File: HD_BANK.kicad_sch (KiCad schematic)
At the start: 1 part, among them J8 DF40HC(3.0)-120DS

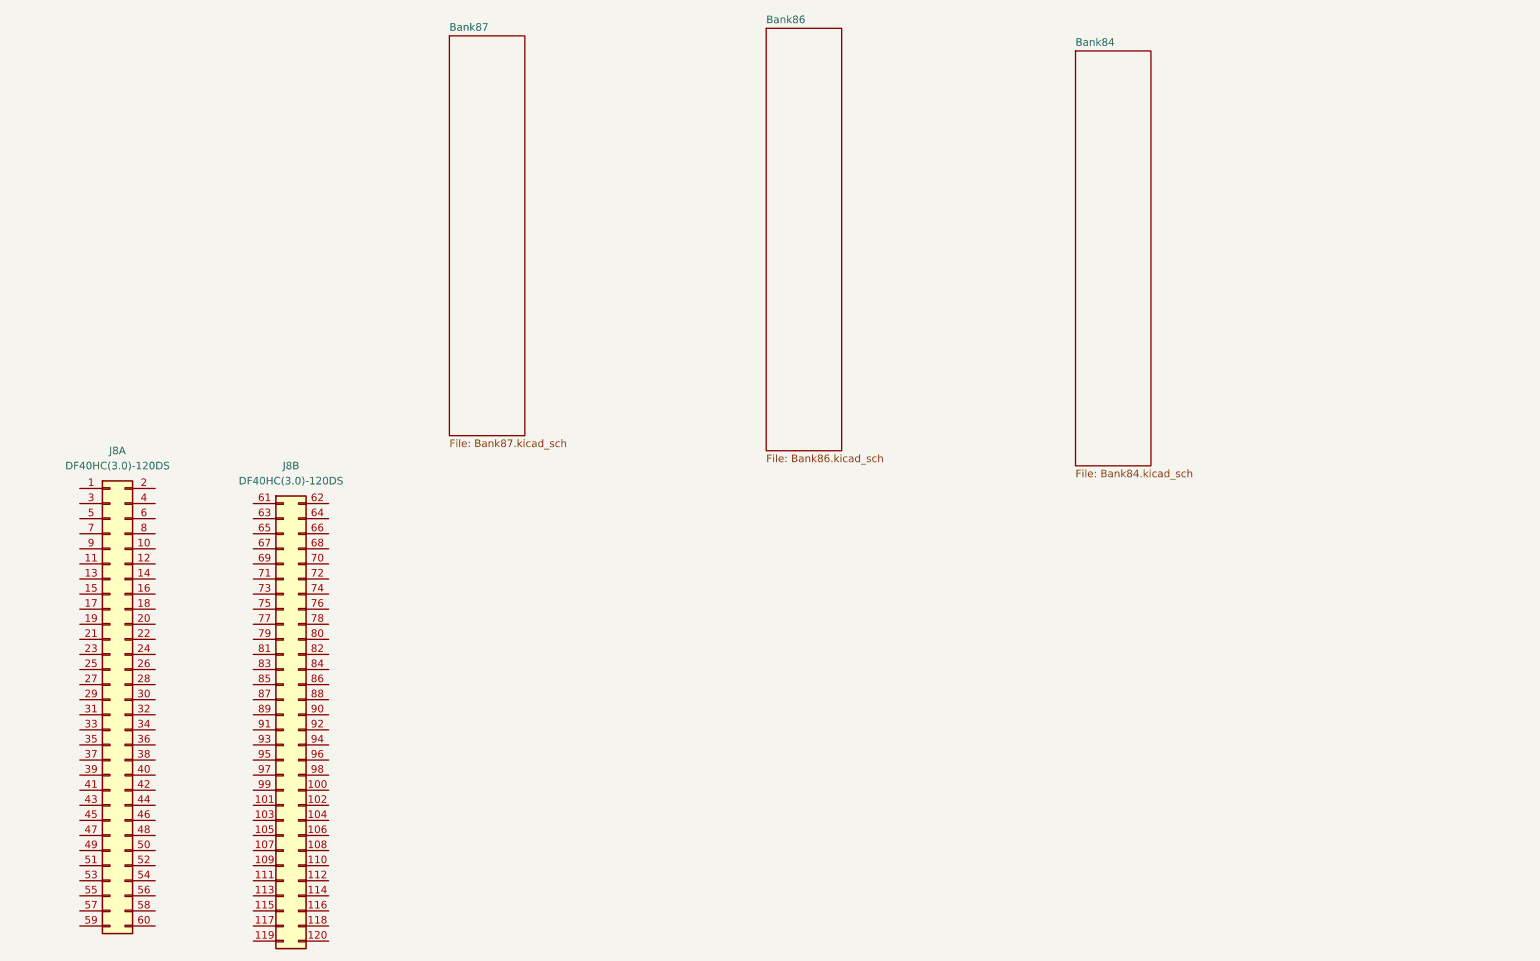
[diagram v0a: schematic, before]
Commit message: finishing schematic
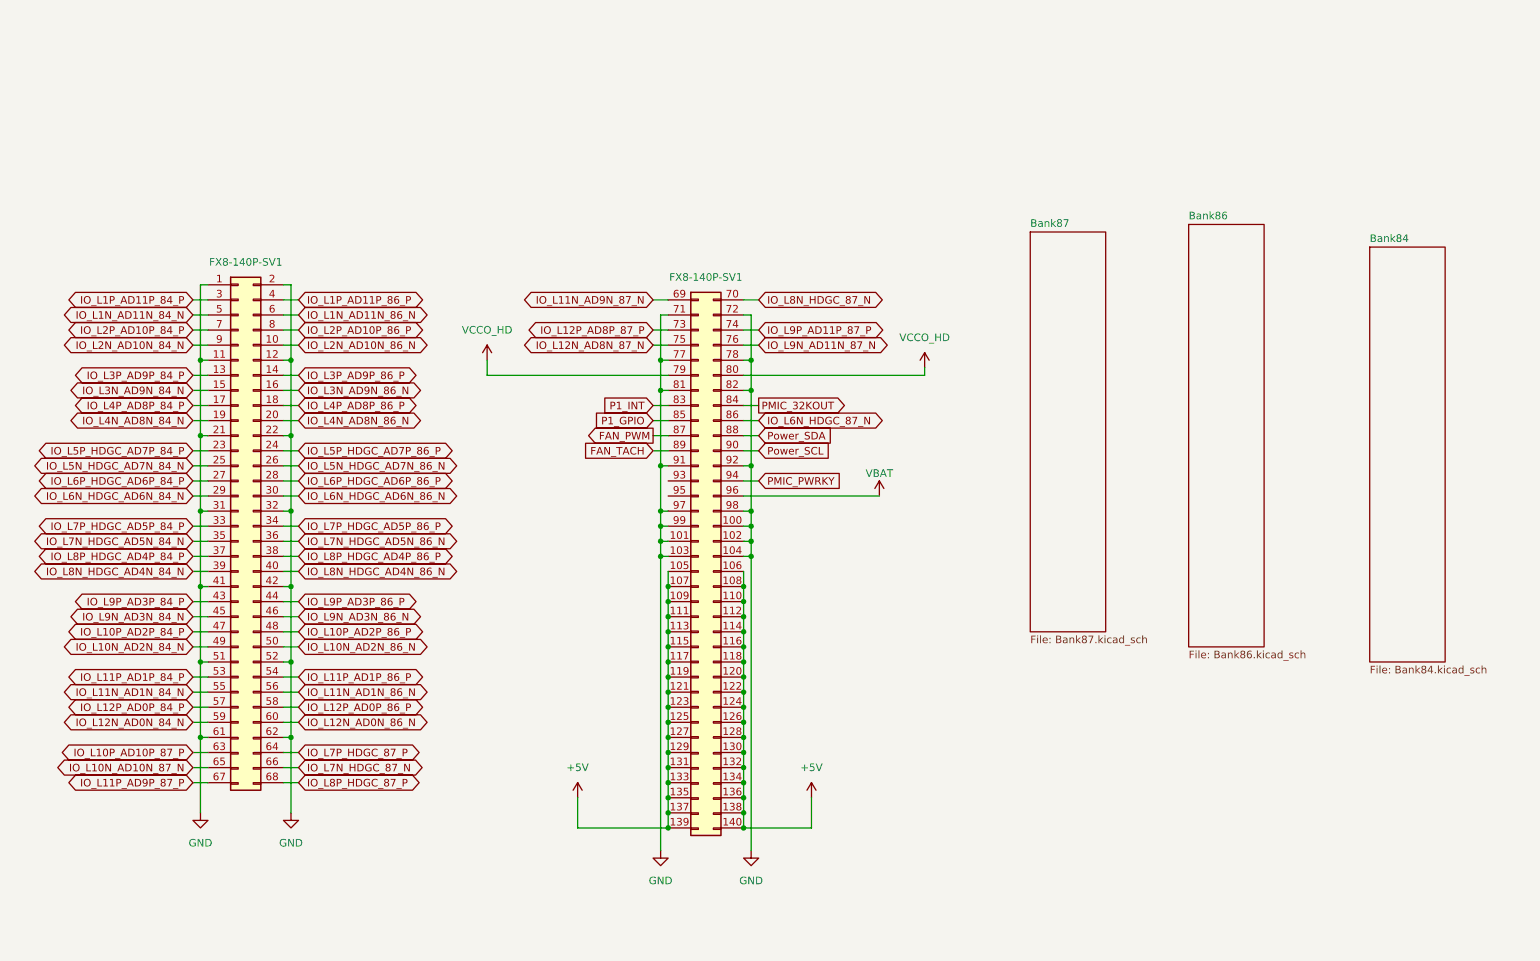
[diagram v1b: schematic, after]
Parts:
- removed J8: DF40HC(3.0)-120DS, Connector_Hirose_DF40:Hirose_DF40C-120DS-0.4V_2x60_P0.4mm, symbol dfdtc_Connector:Conn_02x60_Odd_Even
- added J6: FX8-140P-SV1, Connector_Hirose_FX8:Hirose_FX8-140P-SV_2x70_P0.6mm, symbol dfdtc_Connector:Conn_02x70_Odd_Even
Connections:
- new net +5V: J6.105 (Pin_105), J6.106 (Pin_106), J6.107 (Pin_107), J6.108 (Pin_108), J6.109 (Pin_109), J6.110 (Pin_110), J6.111 (Pin_111), J6.112 (Pin_112), J6.113 (Pin_113), J6.114 (Pin_114), J6.115 (Pin_115), J6.116 (Pin_116), J6.117 (Pin_117), J6.118 (Pin_118), J6.119 (Pin_119), J6.120 (Pin_120), J6.121, J6.122, J6.123, J6.124, J6.125, J6.126, J6.127, J6.128, J6.129, J6.130, J6.131, J6.132, J6.133, J6.134, J6.135, J6.136, J6.137, J6.138, J6.139, J6.140
- new net FAN_PWM: J6.87 (Pin_87)
- new net FAN_TACH: J6.89 (Pin_89)
- new net GND: J6.1 (Pin_1), J6.100 (Pin_100), J6.101 (Pin_101), J6.102 (Pin_102), J6.103 (Pin_103), J6.104 (Pin_104), J6.11 (Pin_11), J6.12 (Pin_12), J6.2 (Pin_2), J6.21 (Pin_21), J6.22 (Pin_22), J6.31 (Pin_31), J6.32 (Pin_32), J6.41 (Pin_41), J6.42 (Pin_42), J6.51 (Pin_51), J6.52 (Pin_52), J6.61 (Pin_61), J6.62 (Pin_62), J6.71 (Pin_71), J6.72 (Pin_72), J6.77 (Pin_77), J6.78 (Pin_78), J6.81 (Pin_81), J6.82 (Pin_82), J6.91 (Pin_91), J6.92 (Pin_92), J6.97 (Pin_97), J6.98 (Pin_98), J6.99 (Pin_99)
- new net IO_L10N_AD10N_87_N: J6.65 (Pin_65)
- new net IO_L10N_AD2N_84_N: J6.49 (Pin_49)
- new net IO_L10N_AD2N_86_N: J6.50 (Pin_50)
- new net IO_L10P_AD10P_87_P: J6.63 (Pin_63)
- new net IO_L10P_AD2P_84_P: J6.47 (Pin_47)
- new net IO_L10P_AD2P_86_P: J6.48 (Pin_48)
- new net IO_L11N_AD1N_84_N: J6.55 (Pin_55)
- new net IO_L11N_AD1N_86_N: J6.56 (Pin_56)
- new net IO_L11N_AD9N_87_N: J6.69 (Pin_69)
- new net IO_L11P_AD1P_84_P: J6.53 (Pin_53)
- new net IO_L11P_AD1P_86_P: J6.54 (Pin_54)
- new net IO_L11P_AD9P_87_P: J6.67 (Pin_67)
- new net IO_L12N_AD0N_84_N: J6.59 (Pin_59)
- new net IO_L12N_AD0N_86_N: J6.60 (Pin_60)
- new net IO_L12N_AD8N_87_N: J6.75 (Pin_75)
- new net IO_L12P_AD0P_84_P: J6.57 (Pin_57)
- new net IO_L12P_AD0P_86_P: J6.58 (Pin_58)
- new net IO_L12P_AD8P_87_P: J6.73 (Pin_73)
- new net IO_L1N_AD11N_84_N: J6.5 (Pin_5)
- new net IO_L1N_AD11N_86_N: J6.6 (Pin_6)
- new net IO_L1P_AD11P_84_P: J6.3 (Pin_3)
- new net IO_L1P_AD11P_86_P: J6.4 (Pin_4)
- new net IO_L2N_AD10N_84_N: J6.9 (Pin_9)
- new net IO_L2N_AD10N_86_N: J6.10 (Pin_10)
- new net IO_L2P_AD10P_84_P: J6.7 (Pin_7)
- new net IO_L2P_AD10P_86_P: J6.8 (Pin_8)
- new net IO_L3N_AD9N_84_N: J6.15 (Pin_15)
- new net IO_L3N_AD9N_86_N: J6.16 (Pin_16)
- new net IO_L3P_AD9P_84_P: J6.13 (Pin_13)
- new net IO_L3P_AD9P_86_P: J6.14 (Pin_14)
- new net IO_L4N_AD8N_84_N: J6.19 (Pin_19)
- new net IO_L4N_AD8N_86_N: J6.20 (Pin_20)
- new net IO_L4P_AD8P_84_P: J6.17 (Pin_17)
- new net IO_L4P_AD8P_86_P: J6.18 (Pin_18)
- new net IO_L5N_HDGC_AD7N_84_N: J6.25 (Pin_25)
- new net IO_L5N_HDGC_AD7N_86_N: J6.26 (Pin_26)
- new net IO_L5P_HDGC_AD7P_84_P: J6.23 (Pin_23)
- new net IO_L5P_HDGC_AD7P_86_P: J6.24 (Pin_24)
- new net IO_L6N_HDGC_87_N: J6.86 (Pin_86)
- new net IO_L6N_HDGC_AD6N_84_N: J6.29 (Pin_29)
- new net IO_L6N_HDGC_AD6N_86_N: J6.30 (Pin_30)
- new net IO_L6P_HDGC_AD6P_84_P: J6.27 (Pin_27)
- new net IO_L6P_HDGC_AD6P_86_P: J6.28 (Pin_28)
- new net IO_L7N_HDGC_87_N: J6.66 (Pin_66)
- new net IO_L7N_HDGC_AD5N_84_N: J6.35 (Pin_35)
- new net IO_L7N_HDGC_AD5N_86_N: J6.36 (Pin_36)
- new net IO_L7P_HDGC_87_P: J6.64 (Pin_64)
- new net IO_L7P_HDGC_AD5P_84_P: J6.33 (Pin_33)
- new net IO_L7P_HDGC_AD5P_86_P: J6.34 (Pin_34)
- new net IO_L8N_HDGC_87_N: J6.70 (Pin_70)
- new net IO_L8N_HDGC_AD4N_84_N: J6.39 (Pin_39)
- new net IO_L8N_HDGC_AD4N_86_N: J6.40 (Pin_40)
- new net IO_L8P_HDGC_87_P: J6.68 (Pin_68)
- new net IO_L8P_HDGC_AD4P_84_P: J6.37 (Pin_37)
- new net IO_L8P_HDGC_AD4P_86_P: J6.38 (Pin_38)
- new net IO_L9N_AD11N_87_N: J6.76 (Pin_76)
- new net IO_L9N_AD3N_84_N: J6.45 (Pin_45)
- new net IO_L9N_AD3N_86_N: J6.46 (Pin_46)
- new net IO_L9P_AD11P_87_P: J6.74 (Pin_74)
- new net IO_L9P_AD3P_84_P: J6.43 (Pin_43)
- new net IO_L9P_AD3P_86_P: J6.44 (Pin_44)
- new net P1_GPIO: J6.85 (Pin_85)
- new net P1_INT: J6.83 (Pin_83)
- new net PMIC_32KOUT: J6.84 (Pin_84)
- new net PMIC_PWRKY: J6.94 (Pin_94)
- new net Power_SCL: J6.90 (Pin_90)
- new net Power_SDA: J6.88 (Pin_88)
- new net VBAT: J6.96 (Pin_96)
- new net VCCO_HD: J6.79 (Pin_79), J6.80 (Pin_80)

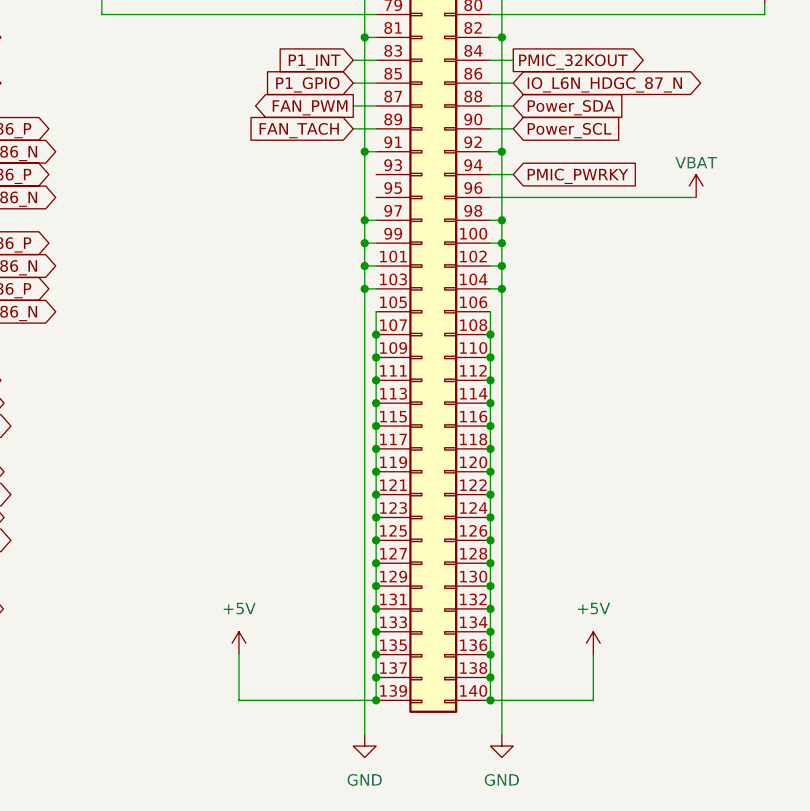
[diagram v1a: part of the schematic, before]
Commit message: sync works
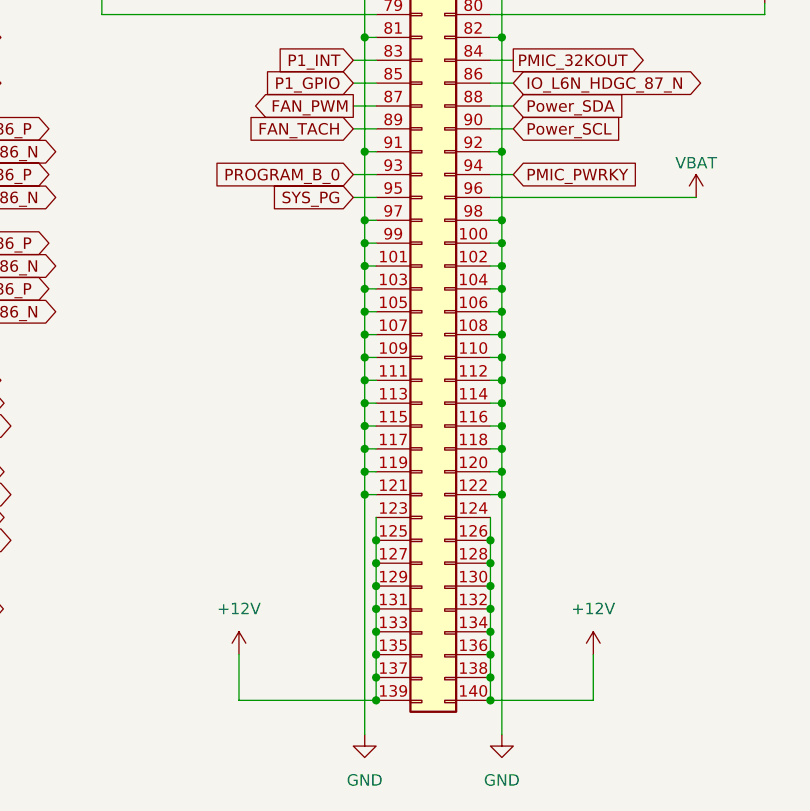
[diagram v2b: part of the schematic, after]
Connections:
- net GND: now also J6.105 (Pin_105), J6.106 (Pin_106), J6.107 (Pin_107), J6.108 (Pin_108), J6.109 (Pin_109), J6.110 (Pin_110), J6.111 (Pin_111), J6.112 (Pin_112), J6.113 (Pin_113), J6.114 (Pin_114), J6.115 (Pin_115), J6.116 (Pin_116), J6.117 (Pin_117), J6.118 (Pin_118), J6.119 (Pin_119), J6.120 (Pin_120), J6.121, J6.122
- net PROGRAM_B_0: now reaches J6.93 (Pin_93)
- net SYS_PG: now reaches J6.95 (Pin_95)
- net +5V renamed +12V
- net +12V: no longer J6.105 (Pin_105), J6.106 (Pin_106), J6.107 (Pin_107), J6.108 (Pin_108), J6.109 (Pin_109), J6.110 (Pin_110), J6.111 (Pin_111), J6.112 (Pin_112), J6.113 (Pin_113), J6.114 (Pin_114), J6.115 (Pin_115), J6.116 (Pin_116), J6.117 (Pin_117), J6.118 (Pin_118), J6.119 (Pin_119), J6.120 (Pin_120), J6.121, J6.122
